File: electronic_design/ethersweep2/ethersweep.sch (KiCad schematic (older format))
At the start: 62 parts, among them J1 AVR-ISP-6, J3 Conn_01x04_Female, J4 Conn_01x02_Male, J5 Conn_01x02_Male, J6 HR911105A, M1 Stepper_Motor_bipolar, SW1 SW_Push, U1 ENC28J60x-SS, U2 ATmega328-AU, U3 DRV8825PWPR, U4 AMS1117-3.3, U5 AS5600, Y1 Crystal_25MHz, Y2 Crystal_8MHz

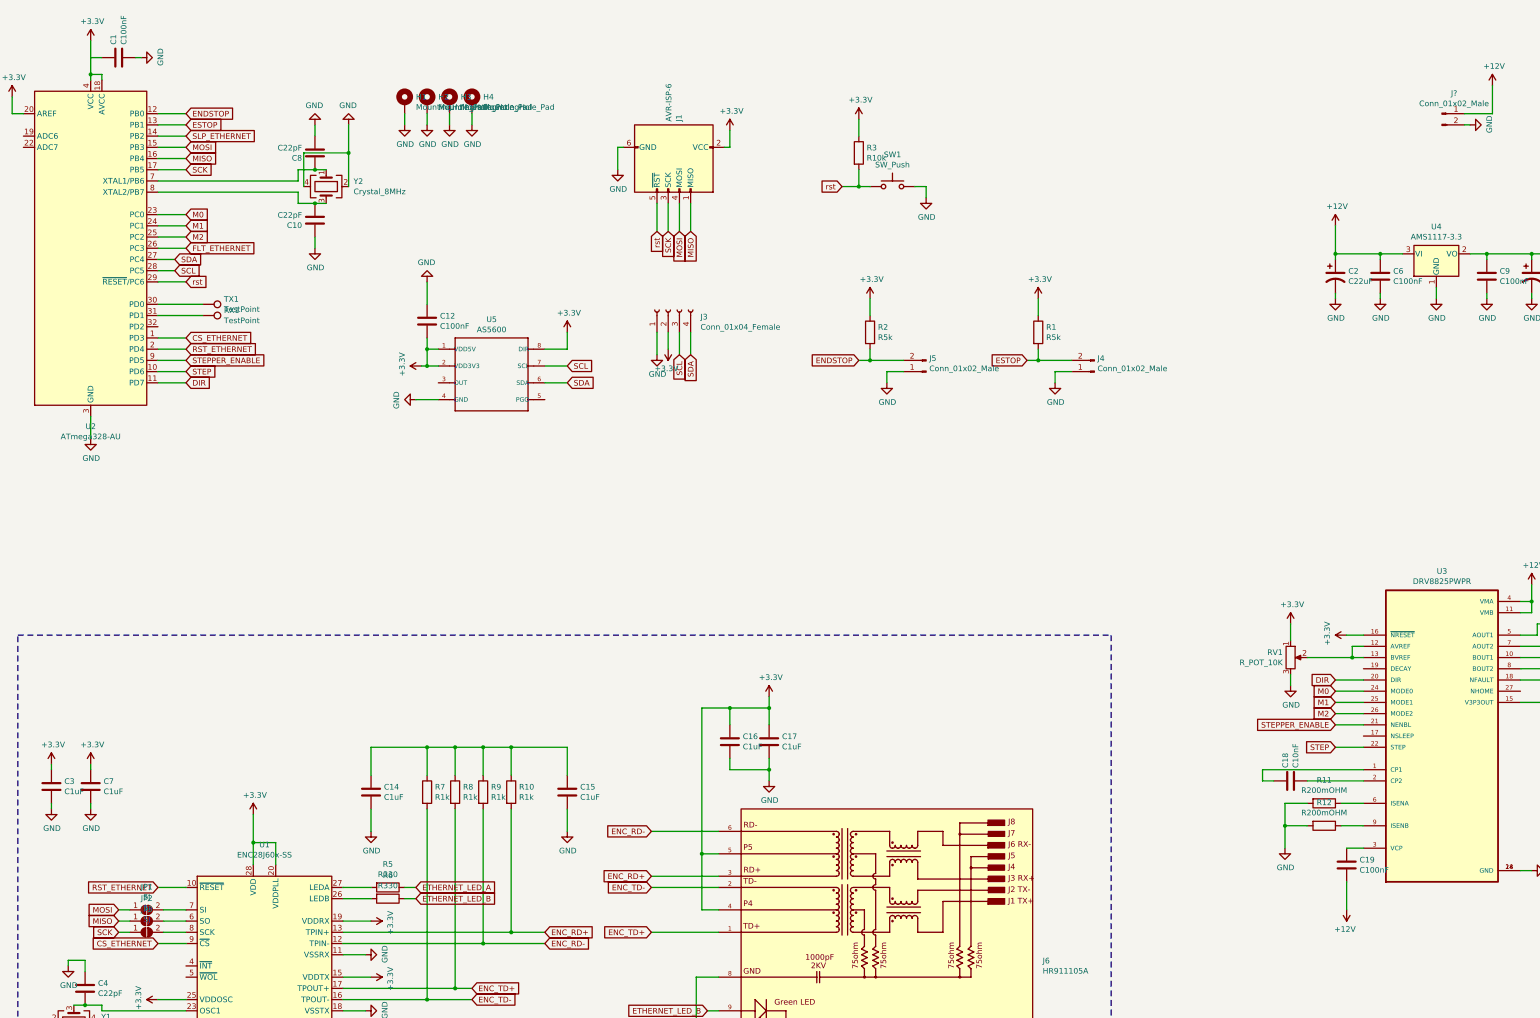
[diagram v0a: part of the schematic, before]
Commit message: raw component layout done
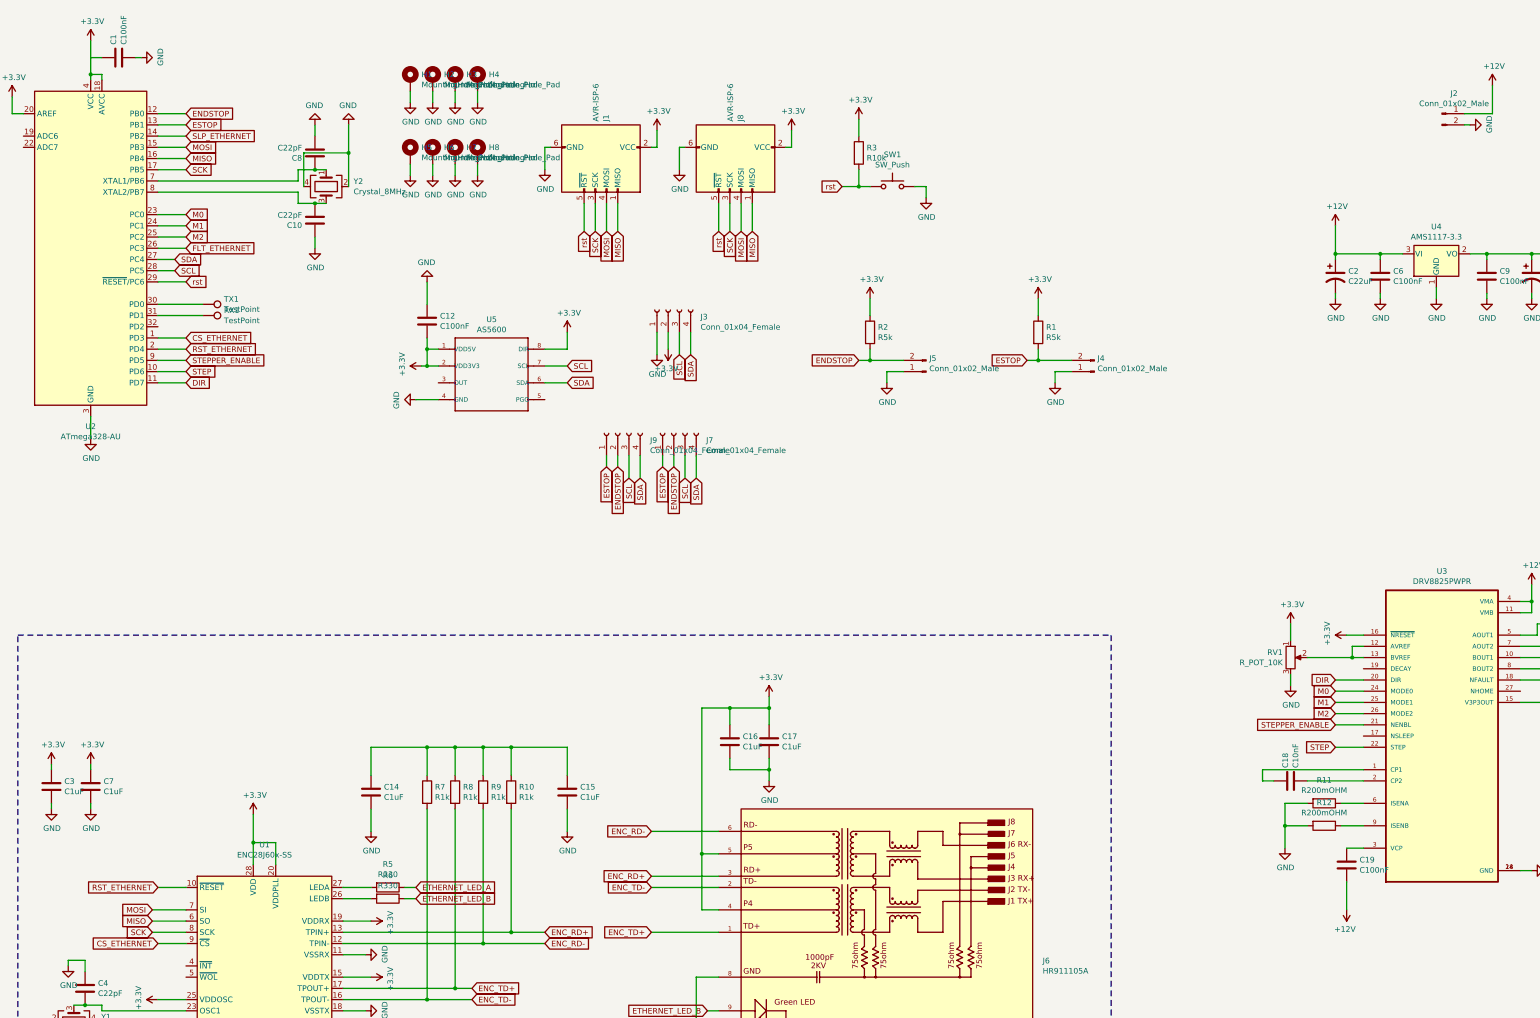
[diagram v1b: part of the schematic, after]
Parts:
- removed JP1, JP2, JP3: SJ, Jumper:SolderJumper-2_P1.3mm_Open_TrianglePad1.0x1.5mm, symbol Jumper:SolderJumper_2_Open
- added H5, H6, H7, H8: MountingHole_Pad, MountingHole:MountingHole_3.2mm_M3_Pad_Via, symbol Mechanical:MountingHole_Pad
- added J7, J9: Conn_01x04_Female, Connector_PinHeader_2.54mm:PinHeader_1x04_P2.54mm_Vertical, symbol Connector:Conn_01x04_Female
- added J8: AVR-ISP-6, Connector_IDC:IDC-Header_2x03_P2.54mm_Vertical, symbol Connector:AVR-ISP-6
- J2: renamed from J?; footprint (none) -> Connector_AMASS:AMASS_XT60-M_1x02_P7.20mm_Vertical
- RX1, TX1: footprint TestPoint:TestPoint_Pad_D3.0mm -> TestPoint:TestPoint_Pad_D2.0mm
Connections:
- net +3V3: now also J8.2 (VCC)
- net ENDSTOP: now also J7.2 (Pin_2), J9.2 (Pin_2)
- net ESTOP: now also J7.1 (Pin_1), J9.1 (Pin_1)
- net GND: now also H5.1, H6.1, H7.1, H8.1, J8.6 (GND)
- net MISO: now also U1.6 (SO), J8.1 (MISO)
- net MOSI: now also U1.7 (SI), J8.4 (MOSI)
- net SCK: now also U1.8 (SCK), J8.3 (SCK)
- net SCL: now also J7.3 (Pin_3), J9.3 (Pin_3)
- net SDA: now also J7.4 (Pin_4), J9.4 (Pin_4)
- net rst: now also J8.5 (~RST)
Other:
- moved on the sheet: H1, H2, H3, H4, J1
